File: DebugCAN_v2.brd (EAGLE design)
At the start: 56 x 63 mm, 58 parts, among them J1 8P8C-LED, J2 XT60PW-M, J3 MA04-1, J4 10118192-0001LF, J5 8P8C-LED, J6 8P8C-LED, J7 8P8C-LED, U1 STM32F302C, U2 NCV7351D1E, U3 SI8621AB-B-IS, U4 AP2127N-3.3TRG1, U5 78L05F, U6 TLP291, X1 CSTCE8M00G55

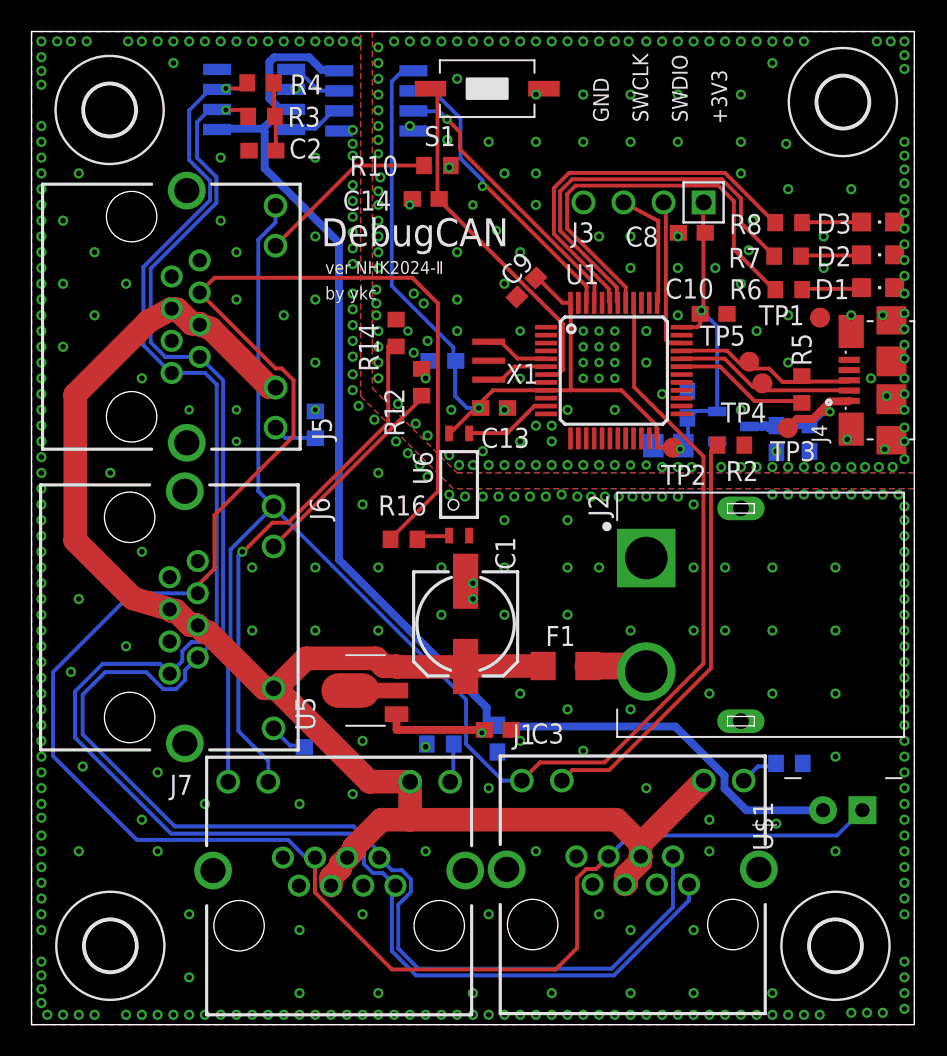
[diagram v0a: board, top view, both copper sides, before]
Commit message: ver.2 update
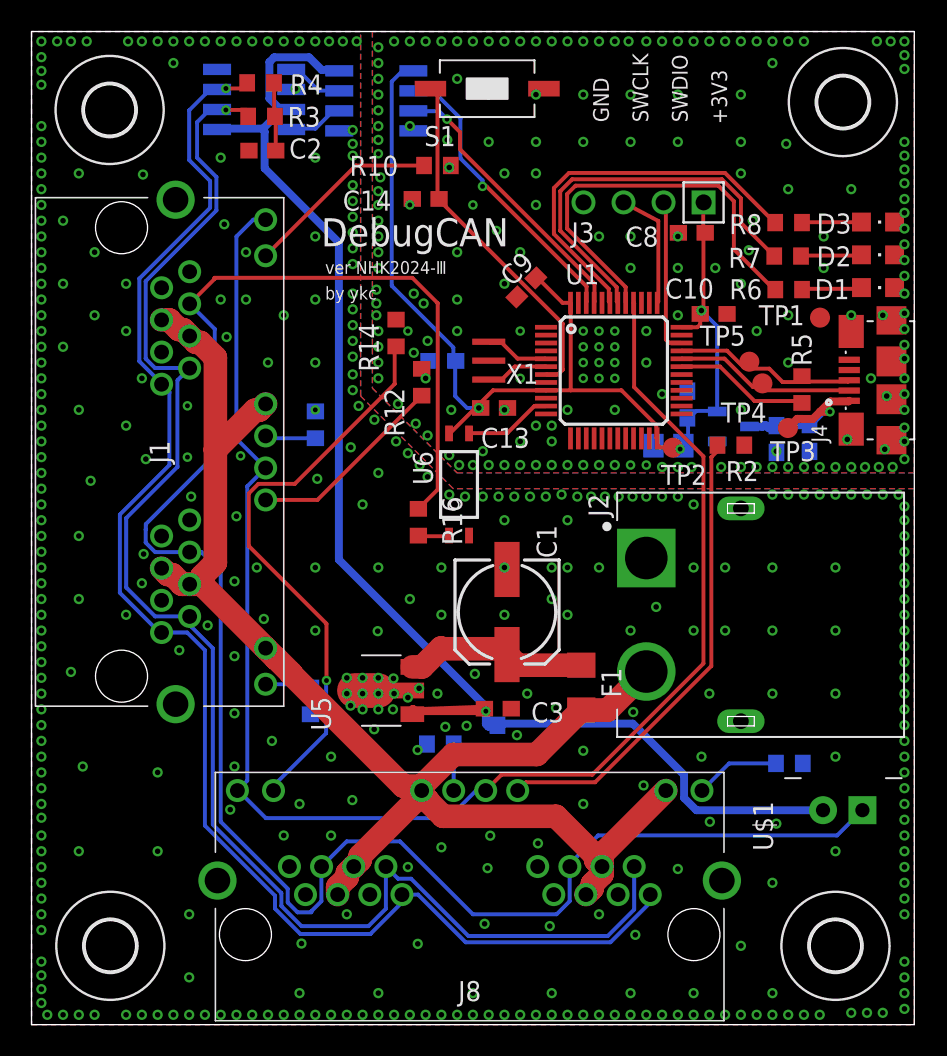
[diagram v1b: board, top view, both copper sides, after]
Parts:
- removed J5, J6, J7: 8P8C-LED, con-rj45:8P8C-LED
- added J8: RJHSE-5381-02, con-rj45:RJHSE538102
- J1: value 8P8C-LED -> RJHSE-5381-02; device con-rj45:8P8C-LED -> con-rj45:RJHSE538102
- moved J1 40.9 mm to (8.25, 40.6), turned to 270 degrees
- moved C1 2.73 mm to (30.2, 26.2)
- moved R11 2.12 mm to (17.7, 20.5), turned to 90 degrees
- moved F1 1.70 mm to (34.9, 21.4), turned to 270 degrees
- moved R16 1.41 mm to (24.5, 31.9), turned to 270 degrees
- moved C3 1.35 mm to (29.6, 20.0)
- moved U5 1.00 mm to (22.2, 21.2)
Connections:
- removed net N$15: J7.YC, R14.2
- new net DCIN: F1.2, J1.A10, J1.A4, J1.A5, J1.B10, J1.B4, J1.B5, J2.2, J8.A10, J8.A4, J8.A5, J8.B10, J8.B4, J8.B5
- net +12V: no longer J1.4, J1.5, J1.GA, J5.4, J5.5, J5.GA, J6.4, J6.5, J6.GA, J7.4, J7.5, J7.GA
- net CANH: now also J1.A1, J1.B1, J8.A1, J8.B1; no longer J1.1, J5.1, J6.1, J7.1
- net CANL: now also J1.A2, J1.B2, J8.A2, J8.B2; no longer J1.2, J5.2, J6.2, J7.2
- net CAN_LED: now also J1.A12, J1.B12, J8.A12, J8.B12; no longer J1.YA, J5.YA, J6.YA, J7.YA
- net EMS: now also J1.A6, J1.B6, J8.A6, J8.B6; no longer J1.6, J5.6, J6.6, J7.6
- net GNDIO: now also J1.A3, J1.A7, J1.A8, J1.B3, J1.B7, J1.B8, J1.MH1, J1.MH2, J8.A3, J8.A7, J8.A8, J8.B3, J8.B7, J8.B8, J8.MH1, J8.MH2; no longer J1.3, J1.7, J1.8, J1.M1, J1.M2, J5.3, J5.7, J5.8, J5.M1, J5.M2, J6.3, J6.7, J6.8, J6.M1, J6.M2, J7.3, J7.7, J7.8, J7.M1, J7.M2
- net N$1: now also J1.A9, R9.2; no longer F1.2, J2.2
- net N$10: now also J1.B11, R12.2; no longer J5.YC, R10.2
- net N$12: now also J1.B9; no longer J6.GC
- net N$13: now also J8.A11, R14.2; no longer J6.YC, R12.2
- net N$14: now also J8.A9; no longer J7.GC
- net N$3: now also J8.B9; no longer J1.GC
- net N$4: now also J8.B11; no longer J1.YC
- net N$9: now also J1.A11, R10.2; no longer J5.GC, R9.2
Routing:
- net DCIN: track 0.00 -> 94.4 mm
- net +12V: track 105.2 -> 11.7 mm
- net N$15: track 33.5 -> 0.00 mm, vias 1 -> 0
- net N$13: track 13.5 -> 36.8 mm, vias 0 -> 1
- net EMS: track 138.3 -> 122.5 mm
- net CANH: track 108.8 -> 93.3 mm
- net CANL: track 108.4 -> 96.8 mm
- net N$9: track 2.83 -> 12.4 mm
- net CAN_LED: track 102.5 -> 98.1 mm
- net +5V_ISO: track 89.3 -> 92.8 mm
- net N$4: track 26.7 -> 29.7 mm
- net N$3: track 2.50 -> 5.41 mm
- net N$10: track 11.5 -> 12.6 mm
- net N$1: track 3.85 -> 3.22 mm
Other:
- board text added: "ver NHK2024-Ⅲ"
- board text removed: "ver NHK2024-Ⅱ"
